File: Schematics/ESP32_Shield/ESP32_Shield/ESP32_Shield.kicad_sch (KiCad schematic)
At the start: 25 parts, among them J1 Conn_01x10, Q1 Si1308EDL, Q3 Si2319CDS, Q4 Si2319CDS, U6 ADS1234IPW, U7 SHT30-DIS

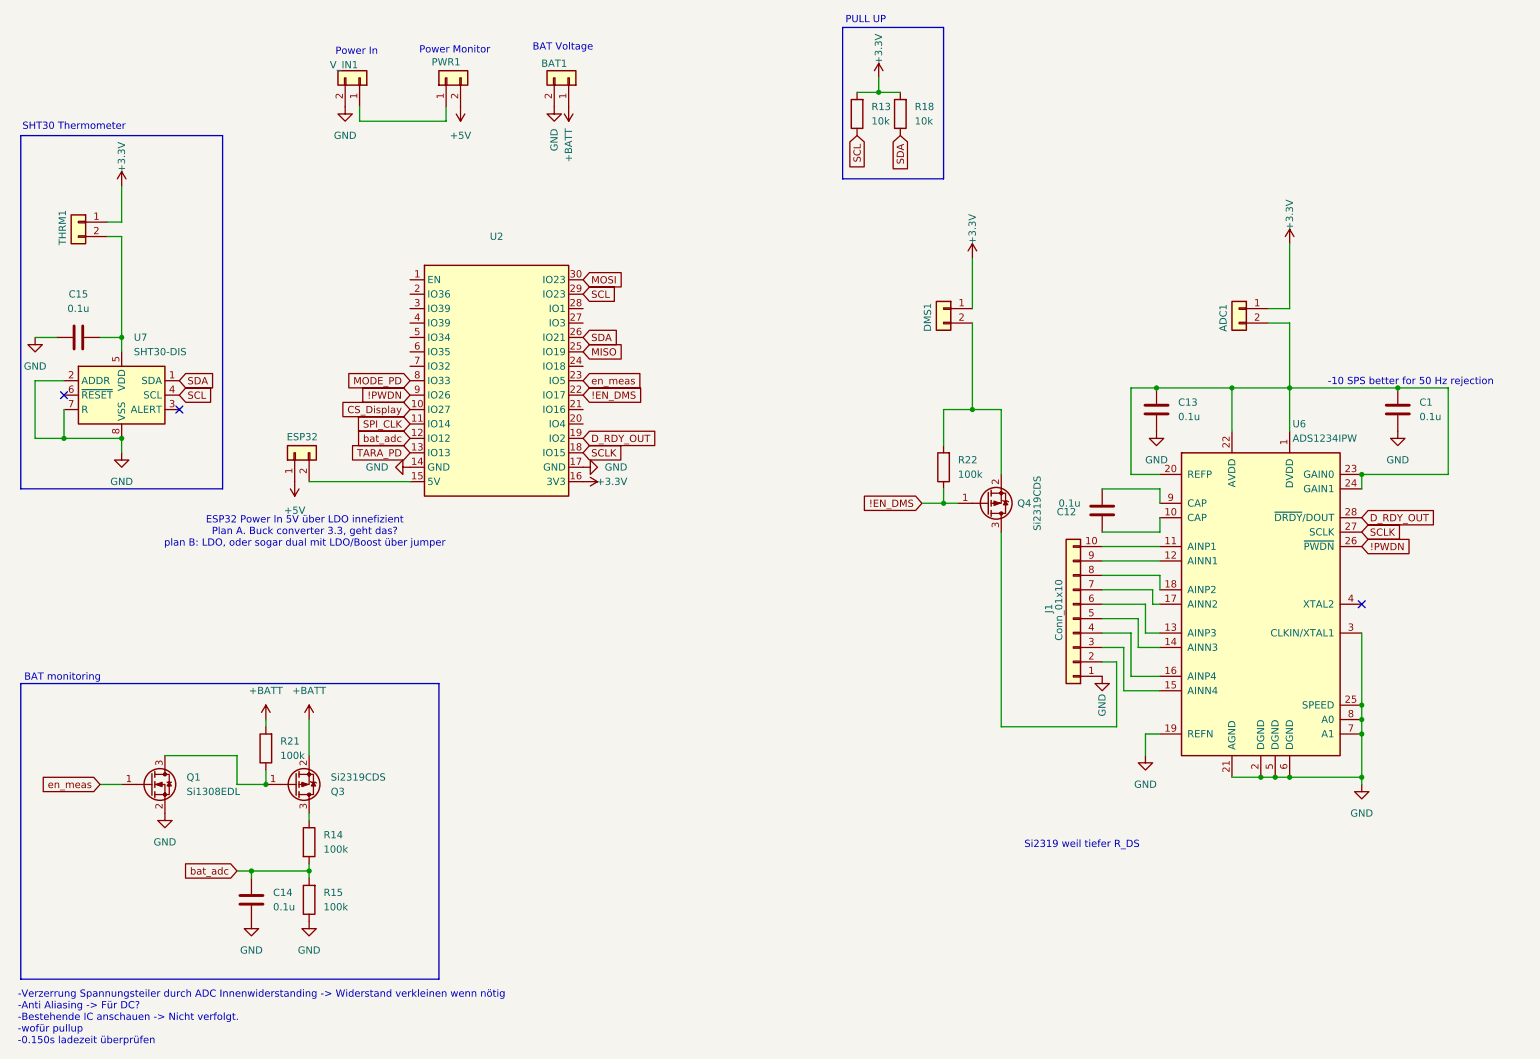
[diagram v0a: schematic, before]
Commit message: a
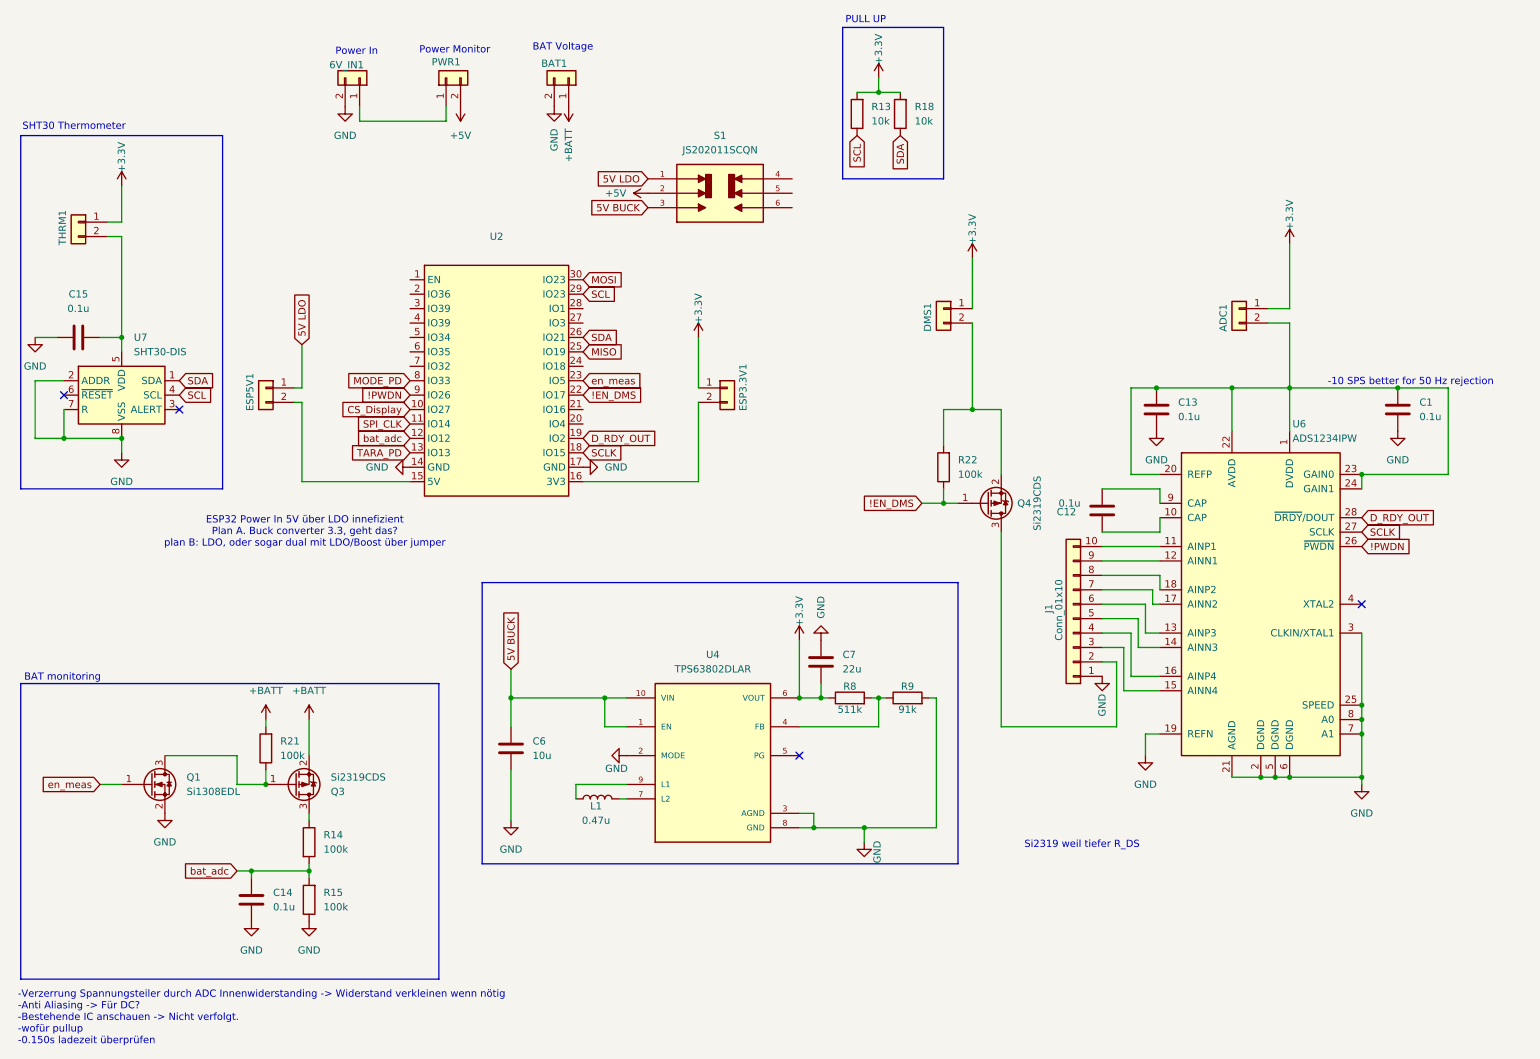
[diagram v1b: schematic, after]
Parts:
- added C6: 10u, Capacitor_SMD:C_0603_1608Metric_Pad1.08x0.95mm_HandSolder, symbol Device:C
- added C7: 22u, Capacitor_SMD:C_0603_1608Metric_Pad1.08x0.95mm_HandSolder, symbol Device:C
- added ESP3.3V1: Conn_01x02, Connector_PinHeader_2.54mm:PinHeader_1x02_P2.54mm_Vertical, symbol Connector_Generic:Conn_01x02
- added L1: 0.47u, Inductor_SMD:L_Coilcraft_XxL4020, symbol Device:L
- added R8: 511k, Resistor_SMD:R_0603_1608Metric_Pad0.98x0.95mm_HandSolder, symbol Device:R
- added R9: 91k, Resistor_SMD:R_0603_1608Metric_Pad0.98x0.95mm_HandSolder, symbol Device:R
- added S1: JS202011SCQN, Button_Switch_SMD:SW_DPDT_CK_JS202011JCQN, symbol JS202011SCQN:JS202011SCQN
- added U4: TPS63802DLAR, TPS63802DLAR:VREG_TPS63802DLAR, symbol TPS63802DLAR:TPS63802DLAR
- renumbered V_IN1 to 6V_IN1, ESP32 to ESP5V1
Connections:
- net +3.3V: now also C7.2, ESP3.3V1.1 (Pin_1), R8.1, U4.6 (VOUT); no longer U2.16 (3V3)
- net +5V: now also S1.2; no longer ESP5V1.1 (Pin_1)
- net GND: now also C6.2, C7.1, R9.2, U4.2 (MODE), U4.3 (AGND), U4.8 (GND)
- new net: R8.2, R9.1, U4.4 (FB)
- new net: L1.2, U4.7 (L2)
- new net: L1.1, U4.9 (L1)
- new net: ESP3.3V1.2 (Pin_2), U2.16 (3V3)
- new net 5V BUCK: C6.1, S1.3, U4.1 (EN), U4.10 (VIN)
- new net 5V LDO: ESP5V1.1 (Pin_1), S1.1
- no-connect marks 3 -> 4
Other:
- moved on the sheet: ESP5V1

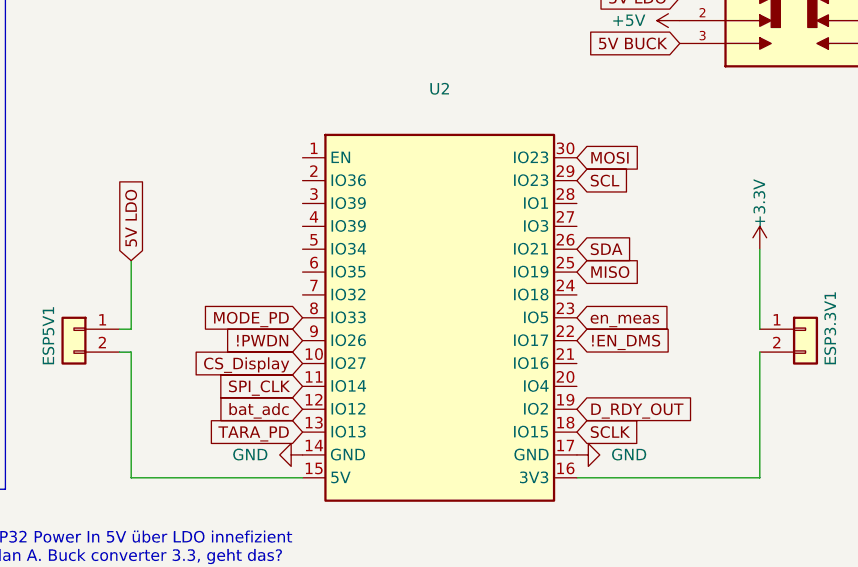
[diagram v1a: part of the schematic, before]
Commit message: l
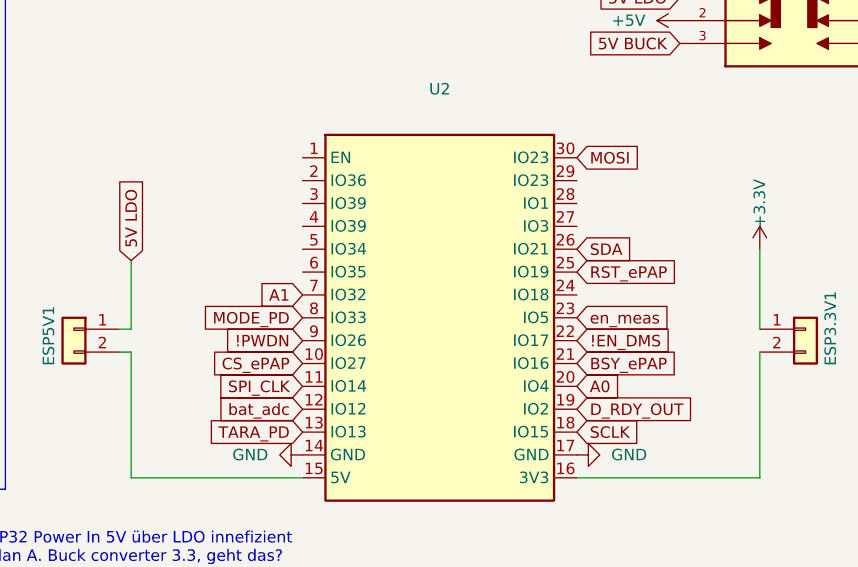
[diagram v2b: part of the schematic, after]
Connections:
- net SCL: no longer U2.29 (IO23)
- net A0: now reaches U2.20 (IO4)
- net BSY_ePAP: now reaches U2.21 (IO16)
- net A1: now reaches U2.7 (IO32)
- net CS_Display renamed CS_ePAP
- net MISO renamed RST_ePAP
